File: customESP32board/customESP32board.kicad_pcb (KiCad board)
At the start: 2 copper layers, 60 x 65 mm, 49 parts, among them J1 USB_B, J2 Conn_01x16_Pin, J3 Conn_01x16_Pin, Q1 S8050, Q2 S8050, Q3 BSS138, Q4 BSS138, Q5 BSS138, SW1 SW_Push, SW2 SW_Push, U1 ESP32-WROOM-32, U2 CH340C, U3 AMS1117-3.3

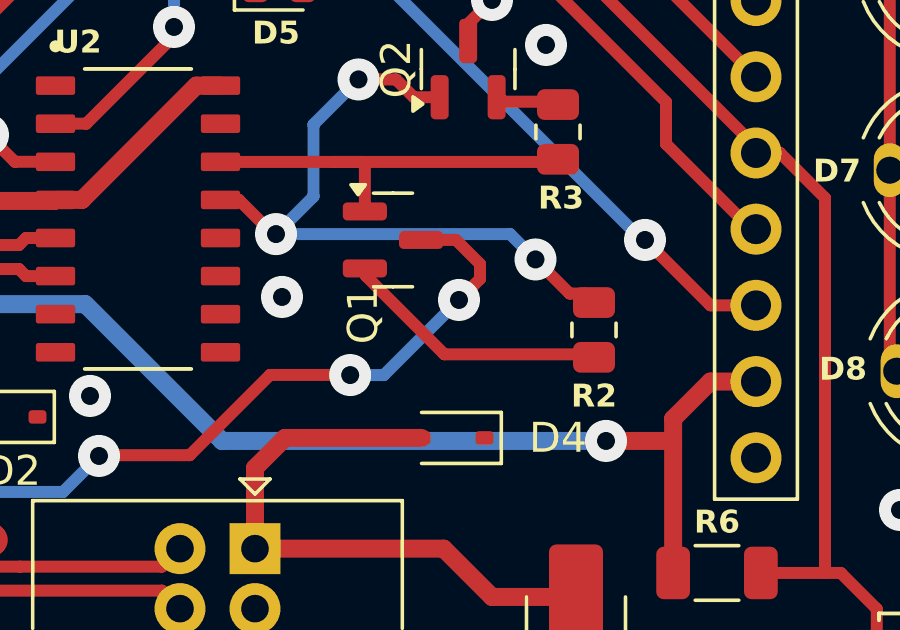
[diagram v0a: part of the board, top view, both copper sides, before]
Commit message: updated routing
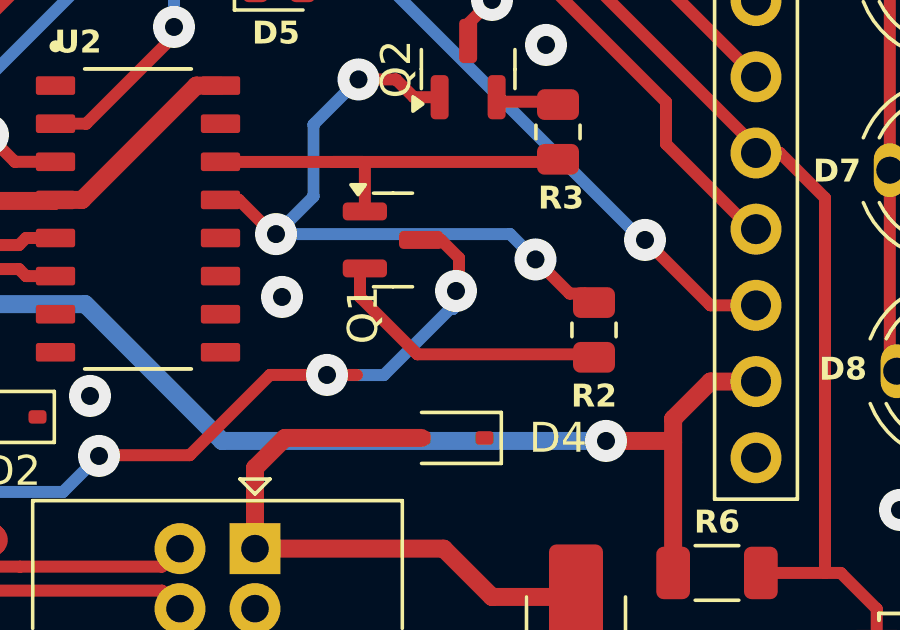
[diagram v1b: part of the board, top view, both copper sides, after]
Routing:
- net Net-(Q1-B): track 8.99 -> 9.65 mm
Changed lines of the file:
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@@
 		(capping no)
 		(filling no)
-		(zone_defaults)
 		(aux_axis_origin 104.5 73.5)
 		(grid_origin 104.5 73.5)
@@
 	)
 	(segment
-		(start 148.6 117.0125)
-		(end 148.5 117.0125)
+		(start 140.8 114.2125)
+		(end 140.9625 114.05)
 		(width 0.4)
 		(layer "F.Cu")
@@
 	)
 	(segment
-		(start 141 114.3)
-		(end 141 114.0875)
+		(start 148.5 117.0125)
+		(end 148.4 116.9125)
 		(width 0.4)
 		(layer "F.Cu")
@@
 	)
 	(segment
-		(start 148.4 116.9125)
-		(end 143.6125 116.9125)
+		(start 142.7125 116.9125)
+		(end 140.8 115)
 		(width 0.4)
 		(layer "F.Cu")
@@
 	)
 	(segment
-		(start 148.5 117.0125)
-		(end 148.4 116.9125)
+		(start 148.4 116.9125)
+		(end 142.7125 116.9125)
 		(width 0.4)
 		(layer "F.Cu")
@@
 	)
 	(segment
-		(start 143.6125 116.9125)
-		(end 141 114.3)
+		(start 148.6 117.0125)
+		(end 148.5 117.0125)
 		(width 0.4)
 		(layer "F.Cu")
@@
 	)
 	(segment
-		(start 141 114.0875)
-		(end 140.9625 114.05)
+		(start 140.8 115)
+		(end 140.8 114.2125)
 		(width 0.4)
 		(layer "F.Cu")
@@
 	)
 	(segment
+		(start 143.5 113.1)
+		(end 142.8375 113.1)
+		(width 0.4)
+		(layer "F.Cu")
+		(net "ESP_EN")
+	)
+	(segment
 		(start 109.1 119.6)
 		(end 108.2375 120.4625)
@@
 	)
 	(segment
+		(start 144 114.8)
+		(end 144 114.5)
+		(width 0.4)
+		(layer "F.Cu")
+		(net "ESP_EN")
+	)
+	(segment
 		(start 108.2375 124.5375)
 		(end 109.6 125.9)
@@
 	)
 	(segment
-		(start 144 113.1)
-		(end 142.8375 113.1)
+		(start 144 114.5)
+		(end 144.1 114.4)
 		(width 0.4)
 		(layer "F.Cu")
@@
 	)
 	(segment
-		(start 144.8 113.9)
-		(end 144 113.1)
+		(start 121.5 82.22)
+		(end 122.2575 82.22)
 		(width 0.4)
 		(layer "F.Cu")
@@
 	)
 	(segment
-		(start 121.5 82.22)
-		(end 122.2575 82.22)
+		(start 144.1 114.4)
+		(end 144.1 113.7)
 		(width 0.4)
 		(layer "F.Cu")
@@
 	)
 	(segment
+		(start 144.1 113.7)
+		(end 143.5 113.1)
+		(width 0.4)
+		(layer "F.Cu")
+		(net "ESP_EN")
+	)
+	(segment
 		(start 108.2375 123)
 		(end 108.2375 124.5375)
@@
 	)
 	(segment
-		(start 144.8 114.4)
-		(end 144.8 113.9)
-		(width 0.4)
-		(layer "F.Cu")
-		(net "ESP_EN")
-	)
-	(segment
 		(start 132.625 120.275)
 		(end 132.6 120.3)
@@
 		(net "ESP_EN")
 	)
-	(segment
-		(start 144.1 115.1)
-		(end 144.8 114.4)
-		(width 0.4)
-		(layer "F.Cu")
-		(net "ESP_EN")
-	)
 	(via
 		(at 132.1 120.3)
@@
 	)
 	(via
-		(at 140.472896 117.60386)
+		(at 139.7 117.6)
 		(size 1.4)
 		(drill 0.6)
@@
 	)
 	(via
-		(at 144.1 115.1)
+		(at 144 114.8)
 		(size 1.4)
 		(drill 0.6)
@@
 	)
 	(segment
+		(start 139.70386 117.60386)
+		(end 139.7 117.6)
+		(width 0.4)
+		(layer "B.Cu")
+		(net "ESP_EN")
+	)
+	(segment
 		(start 109.7 97.4)
 		(end 116.5 90.6)
@@
 	)
 	(segment
+		(start 144 114.8)
+		(end 144 115.3)
+		(width 0.4)
+		(layer "B.Cu")
+		(net "ESP_EN")
+	)
+	(segment
 		(start 121.08 82.22)
 		(end 121.5 82.22)
@@
 	)
 	(segment
-		(start 144.1 115.1)
-		(end 141.59614 117.60386)
+		(start 116.5 90.6)
+		(end 116.5 86.8)
 		(width 0.4)
 		(layer "B.Cu")
@@
 	)
 	(segment
-		(start 116.5 90.6)
-		(end 116.5 86.8)
+		(start 143.8 115.4)
+		(end 141.59614 117.60386)
 		(width 0.4)
 		(layer "B.Cu")
@@
 	)
 	(segment
-		(start 141.59614 117.60386)
-		(end 140.472896 117.60386)
+		(start 109.7 119)
+		(end 109.7 97.4)
 		(width 0.4)
 		(layer "B.Cu")
@@
 	)
 	(segment
-		(start 109.7 119)
-		(end 109.7 97.4)
+		(start 144 115.3)
+		(end 143.9 115.4)
+		(width 0.4)
+		(layer "B.Cu")
+		(net "ESP_EN")
+	)
+	(segment
+		(start 143.9 115.4)
+		(end 143.8 115.4)
 		(width 0.4)
 		(layer "B.Cu")
@@
 		(width 0.4)
 		(layer "B.Cu")
+		(net "ESP_EN")
+	)
+	(segment
+		(start 141.59614 117.60386)
+		(end 139.70386 117.60386)
+		(width 0.4)
+		(layer "B.Cu")
